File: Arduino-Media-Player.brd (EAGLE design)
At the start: 100 x 50 mm, 45 parts, among them J1 MICRO-SD-CARD, U1 ATMEGA328P, U2 FT232RLSSOP, U3 DS1307SO8, U4 AMS117-33, U5 AMS117-18, U6 VS1053B, U7 74HC4050 LVL CONVERTER

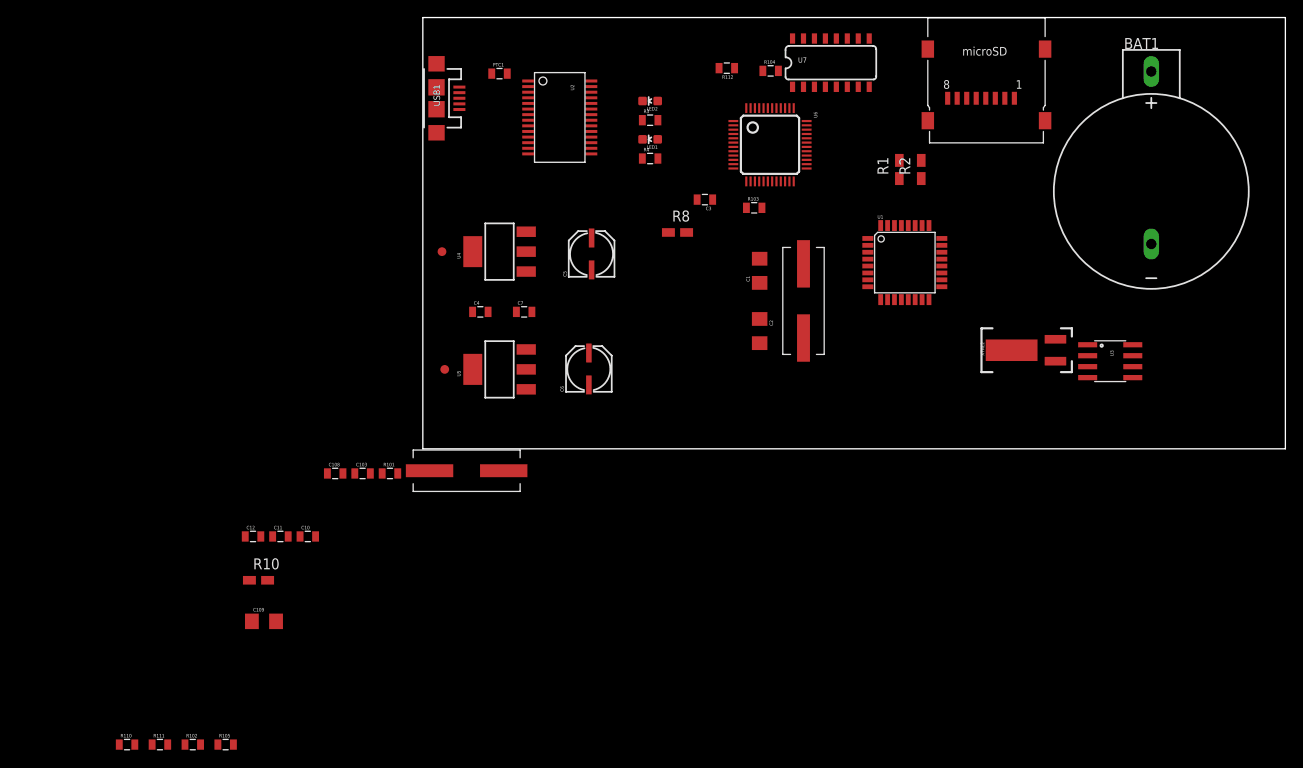
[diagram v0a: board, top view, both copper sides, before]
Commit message: update
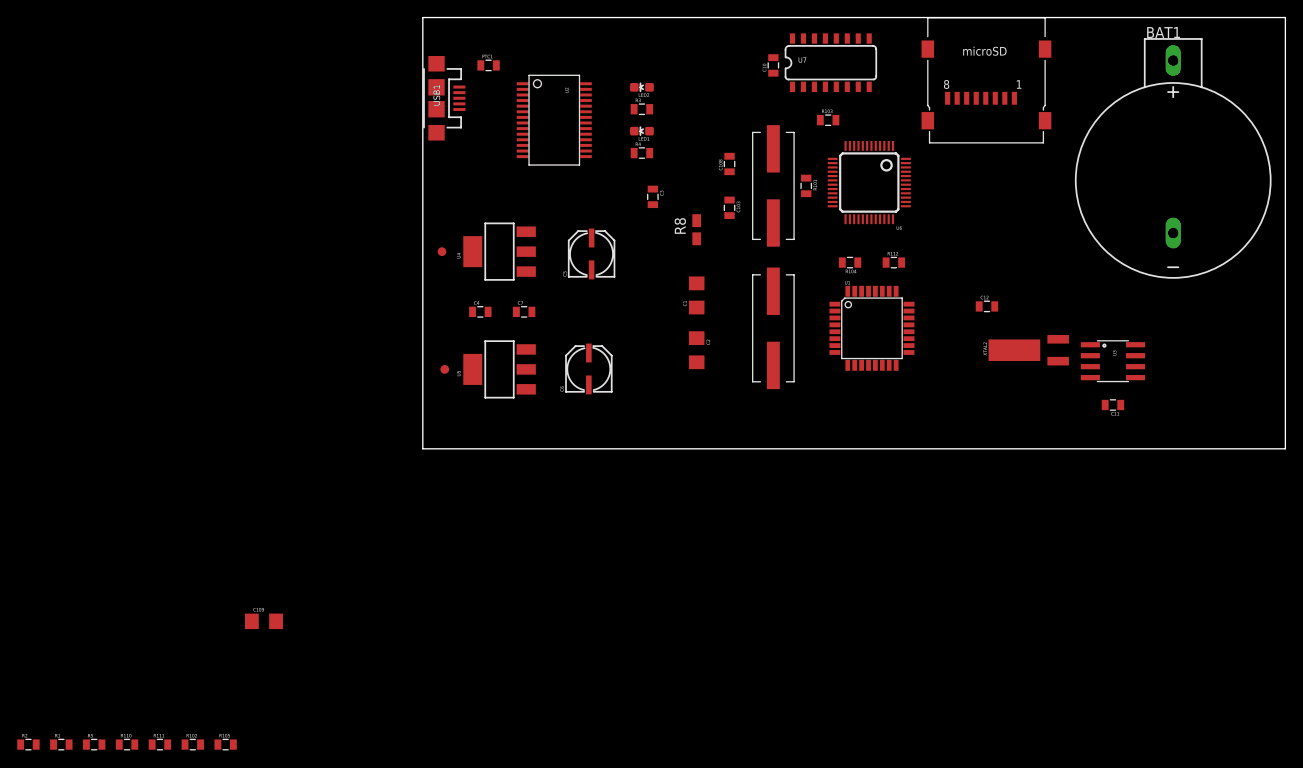
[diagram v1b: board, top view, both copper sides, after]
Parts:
- removed R10: 10K, rcl:R0805W
- added R5: 10K, SparkFun-Passives:0805
- R1, R2: device rcl:R0805W -> SparkFun-Passives:0805
- moved R2 123.1 mm to (-45.7, -34.3), turned to 0 degrees
- moved R1 117.8 mm to (-41.9, -34.3), turned to 0 degrees
- moved C11 97.7 mm to (80.0, 5.08), turned to 180 degrees
- moved C12 89.2 mm to (65.4, 16.5)
- moved C10 76.8 mm to (40.6, 44.5), turned to 90 degrees
- moved R101 58.7 mm to (44.5, 30.5), turned to 270 degrees
- moved C108 58.1 mm to (35.6, 33.0), turned to 90 degrees
- moved C103 52.5 mm to (35.6, 27.9), turned to 270 degrees
- moved XTAL3 48.5 mm to (40.6, 30.5), turned to 270 degrees
- moved R112 29.7 mm to (54.6, 21.6), turned to 0 degrees
- moved R104 24.1 mm to (49.5, 21.6), turned to 180 degrees
- moved R103 13.3 mm to (47.0, 38.1)
- moved U6 12.3 mm to (51.8, 30.9), turned to 180 degrees
- moved U1 8.52 mm to (52.1, 14.0)
- moved C1 7.84 mm to (31.8, 17.8)
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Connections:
- net /RESET: now also R5.1; no longer R10.1
- net 5V: now also R5.2; no longer R10.2
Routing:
- net 3.3V: track 0.00 -> 0.71 mm
